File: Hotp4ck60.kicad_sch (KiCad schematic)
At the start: 46 parts, among them J1 HRO_TYPE-C-31-M-12, SW44 RST, U1 nRF52840, U2 SRV05-4, Y1 32 MHz, Y2 32.768 Khz

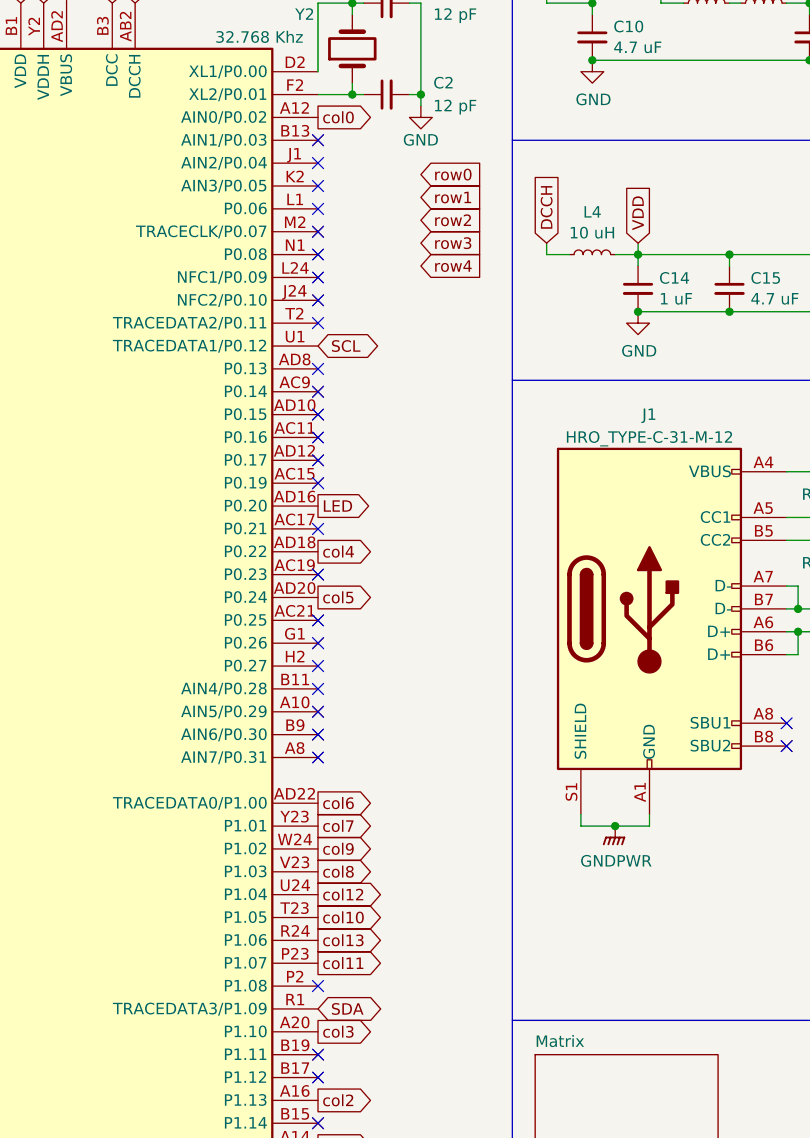
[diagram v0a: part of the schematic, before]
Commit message: Routing finished
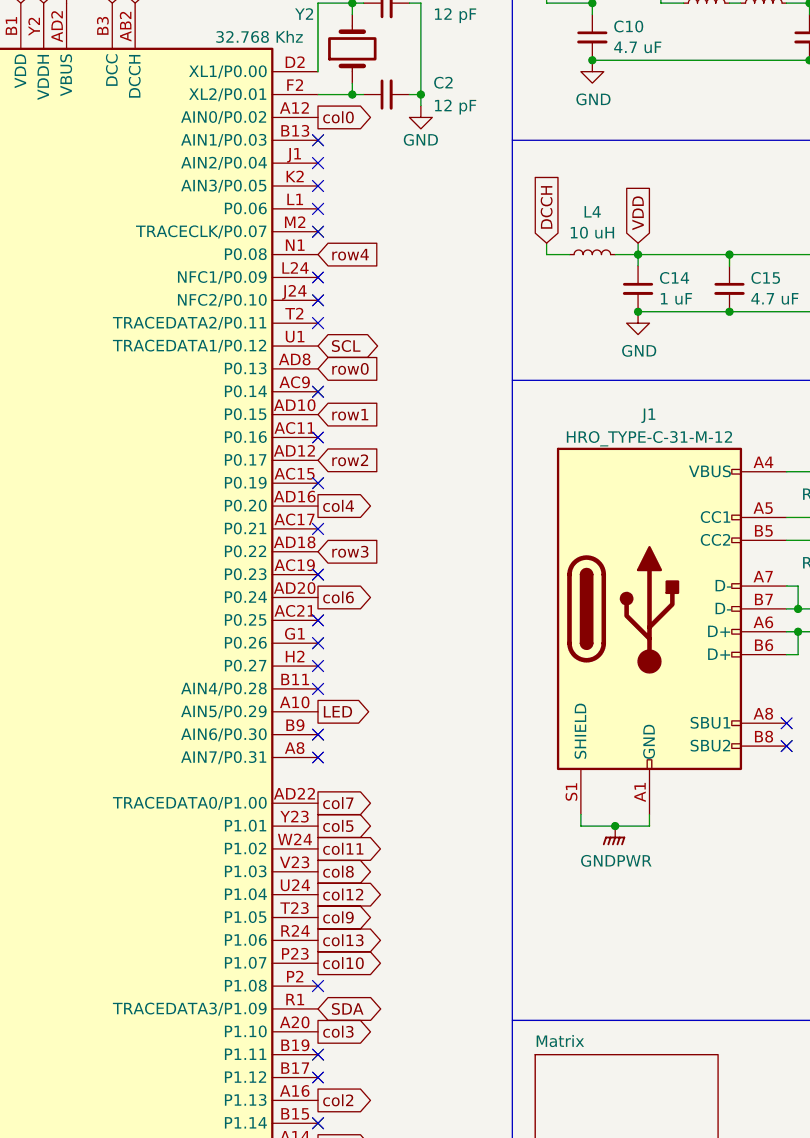
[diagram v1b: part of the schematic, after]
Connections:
- net LED: now also U1.A10 (AIN5/P0.29); no longer U1.AD16 (P0.20)
- net col10: now also U1.P23 (P1.07); no longer U1.T23 (P1.05)
- net col11: now also U1.W24 (P1.02); no longer U1.P23 (P1.07)
- net col4: now also U1.AD16 (P0.20); no longer U1.AD18 (P0.22)
- net col5: now also U1.Y23 (P1.01); no longer U1.AD20 (P0.24)
- net col6: now also U1.AD20 (P0.24); no longer U1.AD22 (TRACEDATA0/P1.00)
- net col7: now also U1.AD22 (TRACEDATA0/P1.00); no longer U1.Y23 (P1.01)
- net col9: now also U1.T23 (P1.05); no longer U1.W24 (P1.02)
- net row0: now also U1.AD8 (P0.13)
- net row1: now also U1.AD10 (P0.15)
- net row2: now also U1.AD12 (P0.17)
- net row3: now also U1.AD18 (P0.22)
- net row4: now also U1.N1 (P0.08)
- no-connect marks 33 -> 28
